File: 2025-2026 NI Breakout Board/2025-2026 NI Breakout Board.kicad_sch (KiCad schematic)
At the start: 205 parts, among them J1 NI9205CONN, J10 GNDCONN, J11 AICONN, J12 AICONN, J13 24VCONN, J14 GNDCONN, J15 NI9205CONN, J16 PWRCONN, J17 24VCONN, J18 GNDCONN, J19 AICONN, J2 PWRCONN, J20 24VCONN, J21 GNDCONN, J22 AICONN, J23 24VCONN, J24 GNDCONN, J25 AICONN, J26 AICONN, J27 24VCONN, J28 GNDCONN, J29 NI9253CONN, J3 24VCONN, J30 AICONN, J31 VSUPCONN, J32 PWRCONN, J33 NI9237CONN, J34 LC0, J35 LC1, J36 LC2, J37 LC3, J38 NI9485CONN, J39 PWRCONN, J4 GNDCONN, J40 AICONN, J41 GNDCONN, J42 NI9485CONN, J43 PWRCONN, J44 AICONN, J45 GNDCONN, J5 AICONN, J6 24VCONN, J7 GNDCONN, J8 AICONN, J9 24VCONN, Q1 FQP27P06, Q2 FQP27P06, Q3 FQP27P06, Q4 FQP27P06, Q5 FQP27P06

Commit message: AGS PCBS
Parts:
- added H10, H11, H12, H13, H14, H15, H16, H17, H18, H19, H20, H21, H22, H23, H24, H25, H26, H27, H28, H29, H30, H7, H8, H9: MountingHole_Pad, MountingHole:MountingHole_3.2mm_M3_DIN965_Pad_TopBottom, symbol Mechanical:MountingHole_Pad
- added J46: NI_9485A_D-SUB, Connector_Dsub:DSUB-9_Pins_Vertical_P2.77x2.84mm_MountingHoles, symbol Connector:DE9_Pins_MountingHoles
- added J47: NI_9485B_D-SUB, Connector_Dsub:DSUB-9_Pins_Vertical_P2.77x2.84mm_MountingHoles, symbol Connector:DE9_Pins_MountingHoles
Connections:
- net EX2+: now also J36.5 (3_1), J36.6 (3_2); no longer J36.7 (4_1), J36.8 (4_2)
- net EX2-: now also J36.7 (4_1), J36.8 (4_2); no longer J36.5 (3_1), J36.6 (3_2)
- net EX3+: now also J37.5 (3_1), J37.6 (3_2); no longer J37.7 (4_1), J37.8 (4_2)
- net EX3-: now also J37.7 (4_1), J37.8 (4_2); no longer J37.5 (3_1), J37.6 (3_2)
- net GND: now also H10.1, H11.1, H12.1, H13.1, H14.1, H15.1, H16.1, H17.1, H18.1, H19.1, H20.1, H21.1, H22.1, H23.1, H24.1, H25.1, H26.1, H27.1, H28.1, H29.1, H30.1, H7.1, H8.1, H9.1, J46.0 (PAD), J46.9, J47.0 (PAD), J47.9
- net NI9237_AI2+: now also J36.10 (5_2), J36.9 (5_1); no longer J36.3 (2_1), J36.4 (2_2)
- net NI9237_AI2-: now also J36.11 (6_1), J36.12 (6_2); no longer J36.1 (1_1), J36.2 (1_2)
- net NI9237_AI3+: now also J37.10 (5_2), J37.9 (5_1); no longer J37.3 (2_1), J37.4 (2_2)
- net NI9237_AI3-: now also J37.11 (6_1), J37.12 (6_2); no longer J37.1 (1_1), J37.2 (1_2)
- net NI9485A_CH0B: now also J46.1
- net NI9485A_CH1B: now also D6.1 (K), R6.1, J46.2
- net NI9485A_CH2B: now also J46.3
- net NI9485A_CH3B: now also J46.4
- net NI9485A_CH4B: now also J46.5
- net NI9485A_CH5B: now also J46.6
- net NI9485A_CH6B: now also J46.7
- net NI9485A_CH7B: now also J46.8
- net NI9485B_CH0B: now also J47.1
- net NI9485B_CH1B: now also J47.2
- net NI9485B_CH2B: now also J47.3
- net NI9485B_CH3B: now also J47.4
- net NI9485B_CH4B: now also J47.5
- net NI9485B_CH5B: now also J47.6
- net NI9485B_CH6B: now also J47.7
- net NI9485B_CH7B: now also J47.8
- net RS2+: now also J36.1 (1_1), J36.2 (1_2); no longer J36.11 (6_1), J36.12 (6_2)
- net RS2-: now also J36.3 (2_1), J36.4 (2_2); no longer J36.10 (5_2), J36.9 (5_1)
- net RS3+: now also J37.1 (1_1), J37.2 (1_2); no longer J37.11 (6_1), J37.12 (6_2)
- net RS3-: now also J37.3 (2_1), J37.4 (2_2); no longer J37.10 (5_2), J37.9 (5_1)
- net V_IN_A: now reaches J39.3 (2_1), J39.4 (2_2), Q4.2 (D)
- net V_IN_B: now reaches J43.3 (2_1), J43.4 (2_2), Q5.2 (D)
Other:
- moved on the sheet: H1, H2, H3, H4, H5, H6, TP1, TP10, TP11, TP12, TP13, TP14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

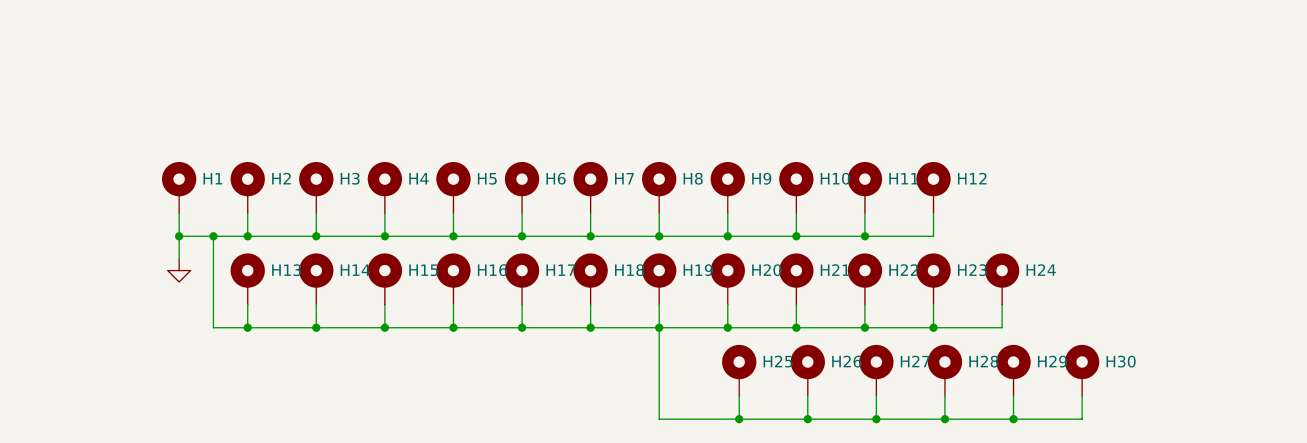
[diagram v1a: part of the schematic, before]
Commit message: Producation files
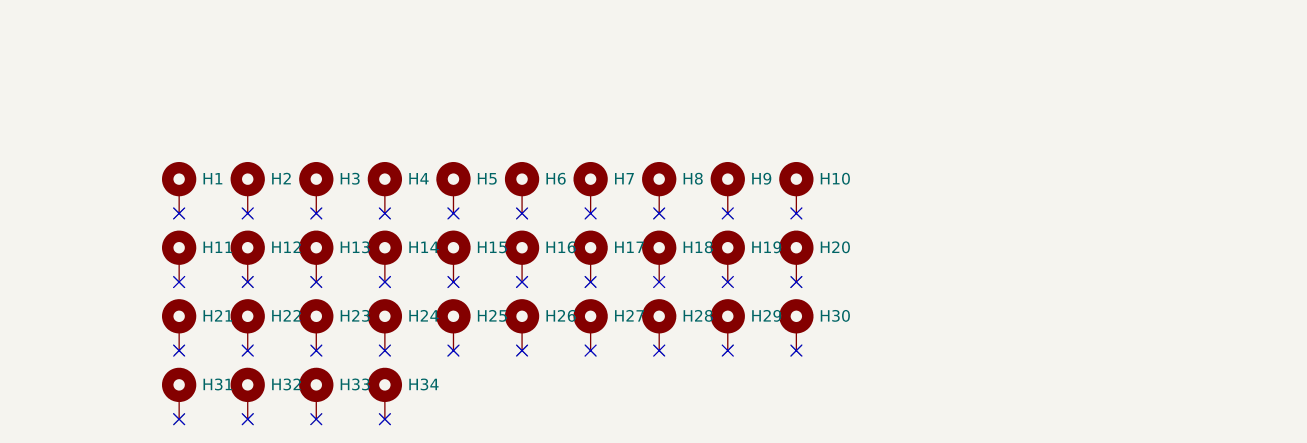
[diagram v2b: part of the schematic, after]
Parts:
- added H31, H32, H33, H34: MountingHole_Pad, MountingHole:MountingHole_3.2mm_M3_DIN965_Pad_TopBottom, symbol Mechanical:MountingHole_Pad
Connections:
- net GND: no longer H1.1, H10.1, H11.1, H12.1, H13.1, H14.1, H15.1, H16.1, H17.1, H18.1, H19.1, H2.1, H20.1, H21.1, H22.1, H23.1, H24.1, H25.1, H26.1, H27.1, H28.1, H29.1, H3.1, H30.1, H4.1, H5.1, H6.1, H7.1, H8.1, H9.1
- no-connect marks 39 -> 73
